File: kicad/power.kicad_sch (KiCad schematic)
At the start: 9 parts, among them J3 Barrel_Jack, U3 TPS62142

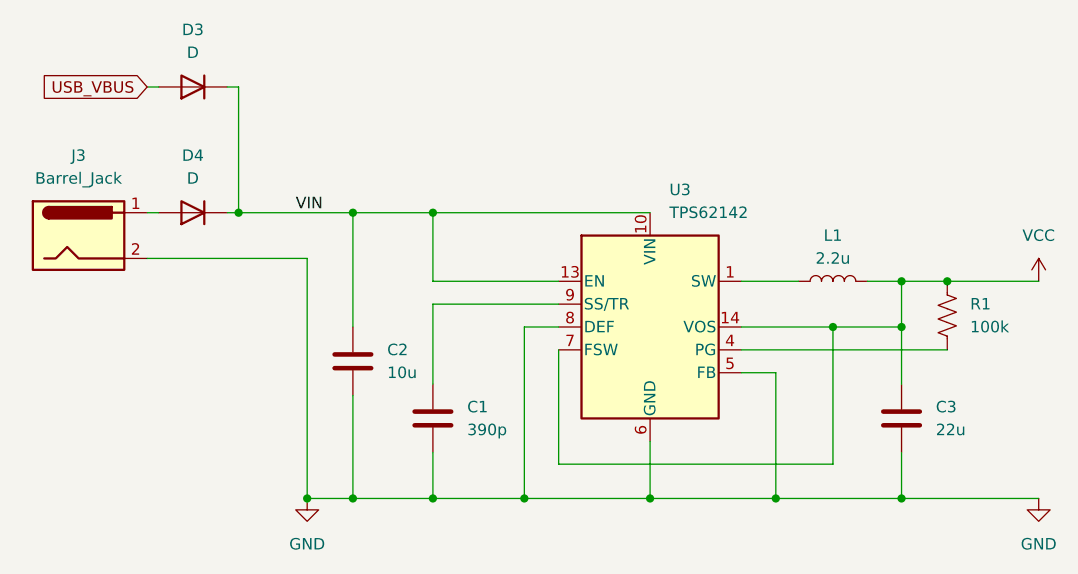
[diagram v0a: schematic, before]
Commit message: Finish basic schematic
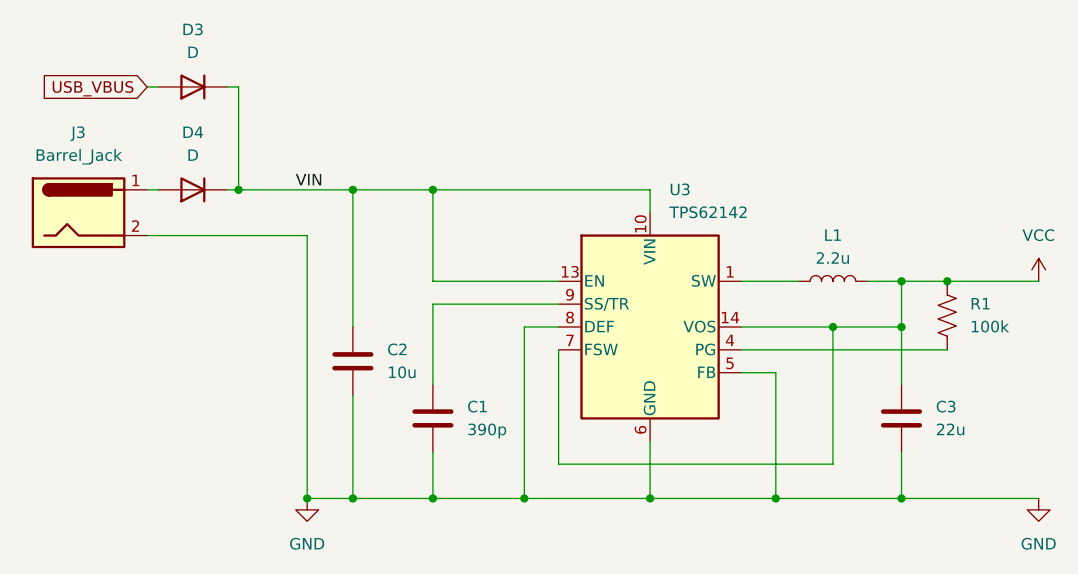
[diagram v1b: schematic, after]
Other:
- moved on the sheet: D4, J3
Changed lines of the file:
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@@
-	)
-	(junction
-		(at 97.79 97.79)
-		(diameter 0)
-		(color 0 0 0 0)
 	)
 	(junction
@@
 	)
 	(junction
-		(at 88.9 97.79)
+		(at 88.9 95.25)
 		(diameter 0)
 		(color 0 0 0 0)
@@
 	)
 	(junction
+		(at 97.79 95.25)
+		(diameter 0)
+		(color 0 0 0 0)
+	)
+	(junction
+		(at 76.2 95.25)
+		(diameter 0)
+		(color 0 0 0 0)
+	)
+	(junction
 		(at 154.94 105.41)
 		(diameter 0)
@@
 	)
 	(junction
-		(at 76.2 97.79)
-		(diameter 0)
-		(color 0 0 0 0)
-	)
-	(junction
 		(at 121.92 129.54)
 		(diameter 0)
@@
 	(wire
 		(pts
-			(xy 66.04 102.87) (xy 83.82 102.87)
+			(xy 66.04 100.33) (xy 83.82 100.33)
 		)
 		(stroke
@@
 	(wire
 		(pts
-			(xy 88.9 97.79) (xy 88.9 110.49)
+			(xy 88.9 95.25) (xy 88.9 110.49)
 		)
 		(stroke
@@
 	(wire
 		(pts
-			(xy 83.82 102.87) (xy 83.82 129.54)
+			(xy 83.82 100.33) (xy 83.82 129.54)
 		)
 		(stroke
@@
 	(wire
 		(pts
-			(xy 97.79 97.79) (xy 97.79 105.41)
+			(xy 97.79 95.25) (xy 97.79 105.41)
+		)
+		(stroke
+			(width 0)
+			(type default)
+		)
+	)
+	(wire
+		(pts
+			(xy 76.2 95.25) (xy 76.2 83.82)
 		)
 		(stroke
@@
 	(wire
 		(pts
-			(xy 97.79 97.79) (xy 121.92 97.79)
+			(xy 97.79 95.25) (xy 121.92 95.25)
 		)
 		(stroke
@@
 	(wire
 		(pts
-			(xy 66.04 97.79) (xy 67.31 97.79)
+			(xy 66.04 95.25) (xy 67.31 95.25)
 		)
 		(stroke
@@
 	(wire
 		(pts
-			(xy 76.2 97.79) (xy 76.2 83.82)
-		)
-		(stroke
-			(width 0)
-			(type default)
-		)
-	)
-	(wire
-		(pts
-			(xy 76.2 97.79) (xy 88.9 97.79)
+			(xy 76.2 95.25) (xy 88.9 95.25)
 		)
 		(stroke
@@
 	(wire
 		(pts
-			(xy 88.9 97.79) (xy 97.79 97.79)
+			(xy 88.9 95.25) (xy 97.79 95.25)
 		)
 		(stroke
@@
 	(wire
 		(pts
-			(xy 74.93 97.79) (xy 76.2 97.79)
+			(xy 74.93 95.25) (xy 76.2 95.25)
 		)
 		(stroke
@@
 	(wire
 		(pts
+			(xy 121.92 95.25) (xy 121.92 97.79)
+		)
+		(stroke
+			(width 0)
+			(type default)
+		)
+	)
+	(wire
+		(pts
 			(xy 97.79 105.41) (xy 111.76 105.41)
 		)
@@
 	)
 	(label "VIN"
-		(at 82.55 97.79 0)
+		(at 82.55 95.25 0)
 		(effects
 			(font
@@
 	(symbol
 		(lib_id "Connector:Barrel_Jack")
-		(at 58.42 100.33 0)
+		(at 58.42 97.79 0)
 		(unit 1)
 		(exclude_from_sim no)
@@
 		(fields_autoplaced yes)
 		(property "Reference" "J3"
+			(at 58.42 88.9 0)
+			(effects
+				(font
+					(size 1.27 1.27)
+				)
+			)
+		)
+		(property "Value" "Barrel_Jack"
 			(at 58.42 91.44 0)
 			(effects
@@
 			)
 		)
-		(property "Value" "Barrel_Jack"
-			(at 58.42 93.98 0)
-			(effects
-				(font
-					(size 1.27 1.27)
-				)
-			)
-		)
 		(property "Footprint" ""
-			(at 59.69 101.346 0)
+			(at 59.69 98.806 0)
 			(effects
 				(font
@@
 		)
 		(property "Datasheet" "~"
-			(at 59.69 101.346 0)
+			(at 59.69 98.806 0)
 			(effects
 				(font
@@
 		)
 		(property "Description" "DC Barrel Jack"
-			(at 58.42 100.33 0)
+			(at 58.42 97.79 0)
 			(effects
 				(font
@@
 	(symbol
 		(lib_id "Device:D")
-		(at 71.12 97.79 180)
+		(at 71.12 95.25 180)
 		(unit 1)
 		(exclude_from_sim no)
@@
 		(fields_autoplaced yes)
 		(property "Reference" "D4"
+			(at 71.12 88.9 0)
+			(effects
+				(font
+					(size 1.27 1.27)
+				)
+			)
+		)
+		(property "Value" "D"
 			(at 71.12 91.44 0)
 			(effects
@@
 			)
 		)
-		(property "Value" "D"
-			(at 71.12 93.98 0)
-			(effects
-				(font
-					(size 1.27 1.27)
-				)
-			)
-		)
 		(property "Footprint" ""
-			(at 71.12 97.79 0)
+			(at 71.12 95.25 0)
 			(effects
 				(font
@@
 		)
 		(property "Datasheet" "~"
-			(at 71.12 97.79 0)
+			(at 71.12 95.25 0)
 			(effects
 				(font
@@
 		)
 		(property "Description" "Diode"
-			(at 71.12 97.79 0)
+			(at 71.12 95.25 0)
 			(effects
 				(font
@@
 		)
 		(property "Sim.Device" "D"
-			(at 71.12 97.79 0)
+			(at 71.12 95.25 0)
 			(effects
 				(font
@@
 		)
 		(property "Sim.Pins" "1=K 2=A"
-			(at 71.12 97.79 0)
-			(effects
-				(font
+			(at 71.12 95.25 0)
+			(effects
+				(font
